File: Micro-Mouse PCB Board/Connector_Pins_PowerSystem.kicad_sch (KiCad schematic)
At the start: 1 part, among them J1 Conn_02x16_Odd_Even

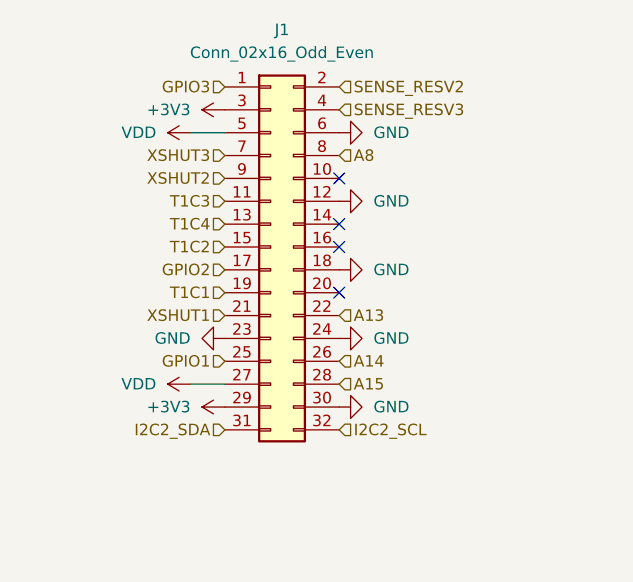
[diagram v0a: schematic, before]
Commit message: Latest Files
v1.0 of Micro-Mouse PCB Design
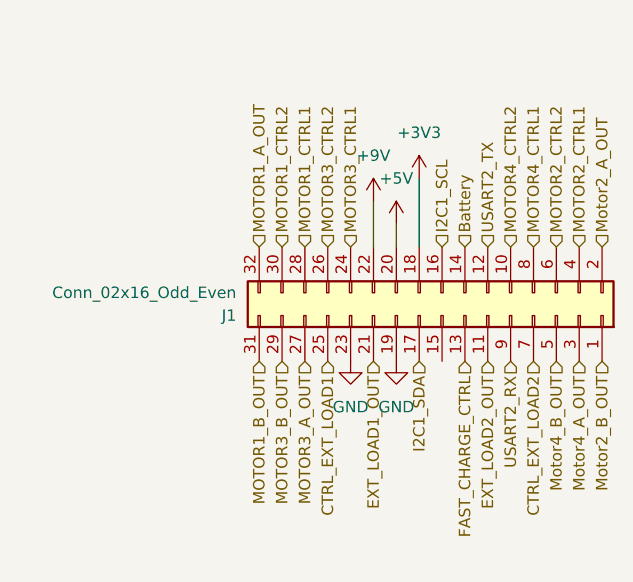
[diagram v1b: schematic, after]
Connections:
- net T1C1 is gone; now on net GND: J1.19 (Pin_19)
- net +3V3: now also J1.18 (Pin_18); no longer J1.29 (Pin_29), J1.3 (Pin_3)
- net GND: no longer J1.12 (Pin_12), J1.18 (Pin_18), J1.24 (Pin_24), J1.30 (Pin_30), J1.6 (Pin_6)
- net MOTOR4_CTRL2: now reaches J1.10 (Pin_10)
- net Battery: now reaches J1.14 (Pin_14)
- net I2C1_SCL: now reaches J1.16 (Pin_16)
- net +5V: now reaches J1.20 (Pin_20)
- net A13 renamed +9V
- net A14 renamed MOTOR3_CTRL2
- net A15 renamed MOTOR1_CTRL1
- net A8 renamed MOTOR4_CTRL1
- net GPIO1 renamed CTRL_EXT_LOAD1
- net GPIO2 renamed I2C1_SDA
- net GPIO3 renamed Motor2_B_OUT
- net I2C2_SCL renamed MOTOR1_A_OUT
- net I2C2_SDA renamed MOTOR1_B_OUT
- net SENSE_RESV2 renamed Motor2_A_OUT
- net SENSE_RESV3 renamed MOTOR2_CTRL1
- net T1C2: no longer names the net of J1.15 (Pin_15)
- net T1C3 renamed EXT_LOAD2_OUT
- net T1C4 renamed FAST_CHARGE_CTRL
- net VDD renamed MOTOR3_A_OUT
- net MOTOR3_A_OUT: no longer J1.5 (Pin_5)
- net XSHUT1 renamed EXT_LOAD1_OUT
- net XSHUT2 renamed USART2_RX
- net XSHUT3 renamed CTRL_EXT_LOAD2
- new net MOTOR1_CTRL2: J1.30 (Pin_30)
- new net MOTOR2_CTRL2: J1.6 (Pin_6)
- new net MOTOR3_B_OUT: J1.29 (Pin_29)
- new net MOTOR3_CTRL1: J1.24 (Pin_24)
- new net Motor4_A_OUT: J1.3 (Pin_3)
- new net Motor4_B_OUT: J1.5 (Pin_5)
- new net USART2_TX: J1.12 (Pin_12)
- no-connect marks 4 -> 0
